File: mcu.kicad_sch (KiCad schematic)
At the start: 44 parts, among them Q1 BC847, SW1 SW_Push, U1 STM32H562RITx, Y2 24 Mhz

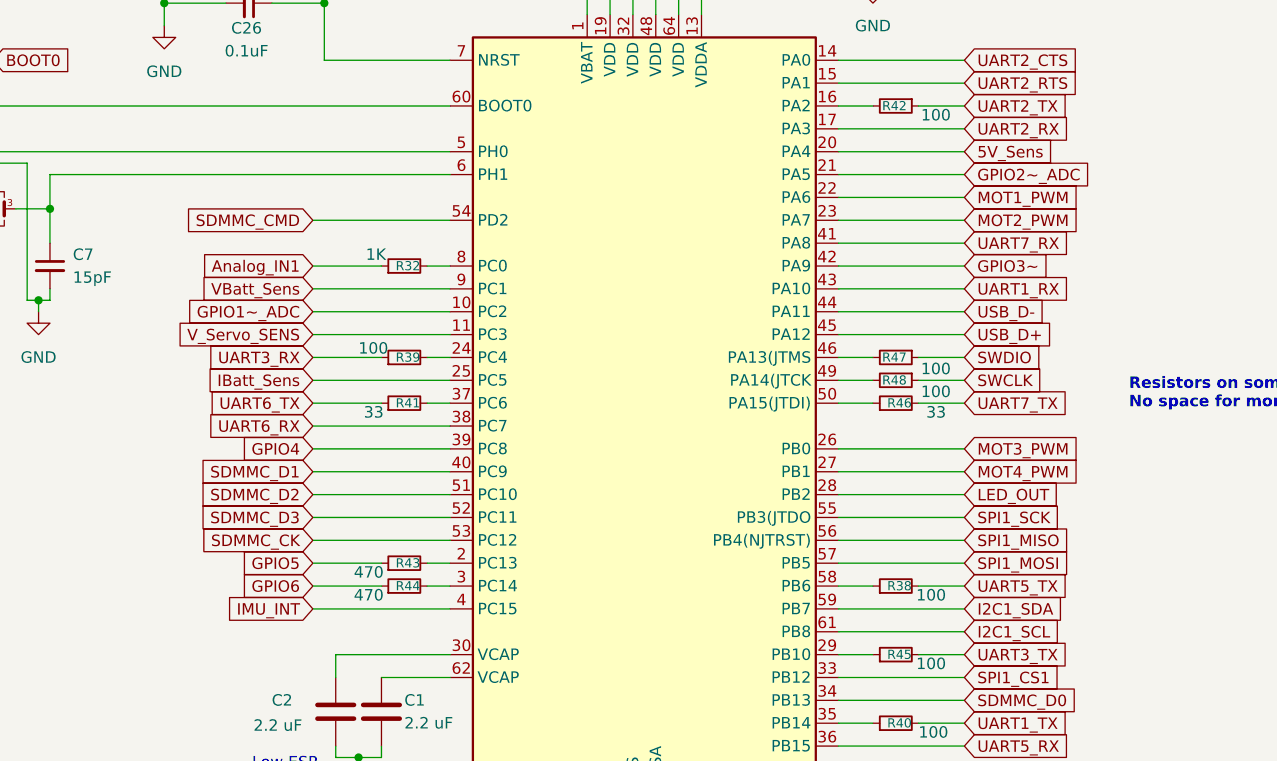
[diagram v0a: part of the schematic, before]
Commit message: Add V1.1
Add V1.1

Add V1.1
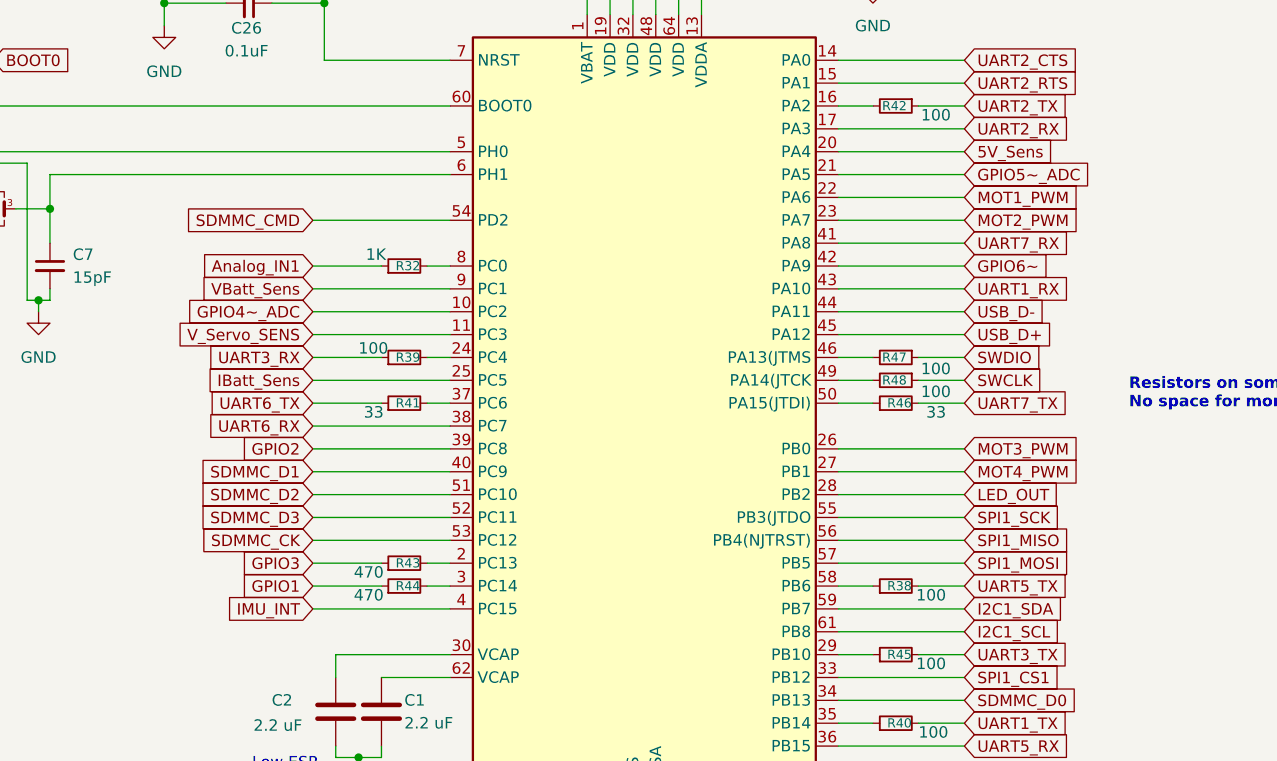
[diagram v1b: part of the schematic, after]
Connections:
- net GPIO1~_ADC renamed GPIO4~_ADC
- net GPIO2~_ADC renamed GPIO5~_ADC
- net GPIO3~ renamed GPIO6~
- net GPIO4 renamed GPIO2
- net GPIO5 renamed GPIO3
- net GPIO6 renamed GPIO1
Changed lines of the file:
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@@
 	(title_block
 		(title "STM32H5 FC")
-		(date "08/06/2026")
-		(rev "v1")
+		(date "2026-05-11")
+		(rev "v1.1")
 		(comment 1 "Evans Cesil Thomas")
 	)
